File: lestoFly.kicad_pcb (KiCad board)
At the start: 2 copper layers, 23 x 29 mm, 24 parts, among them J1 Conn_01x02_Male, J2 Conn_01x15_Male, J5 Conn_Coaxial, U1 ESP32-WROOM-32D, U2 LMZM23601V3, U3 BMP280, U4 RFM95W-868S2, U5 BMX160

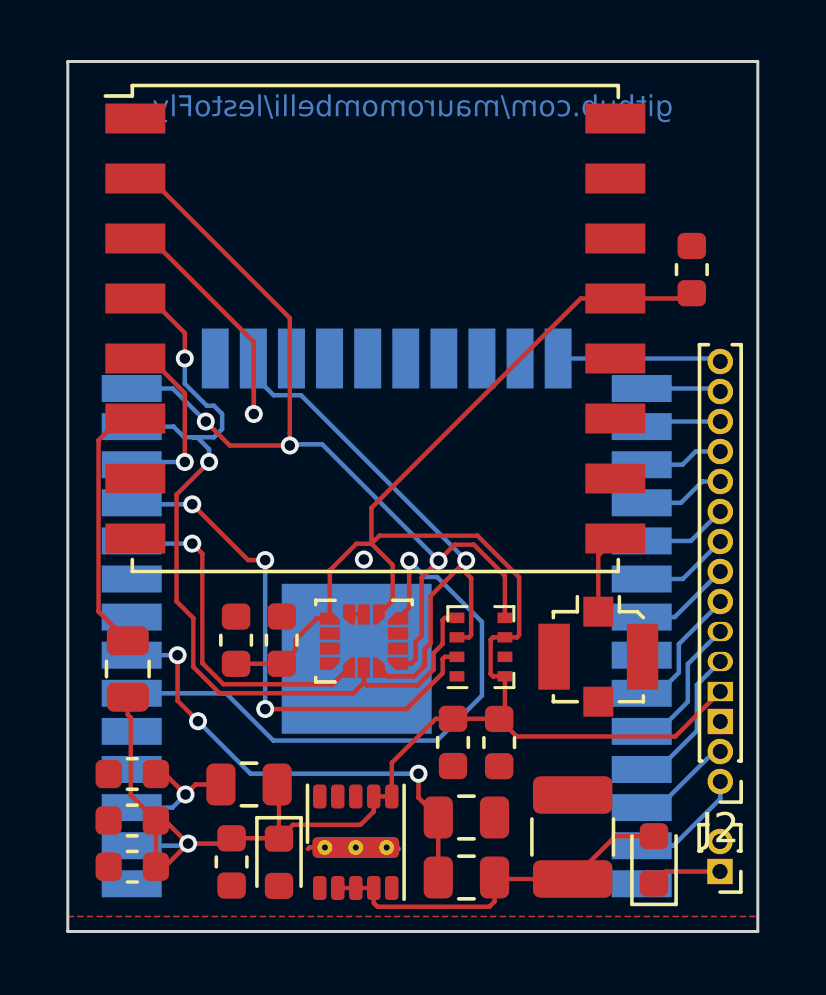
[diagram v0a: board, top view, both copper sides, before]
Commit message: completed the esp32 version
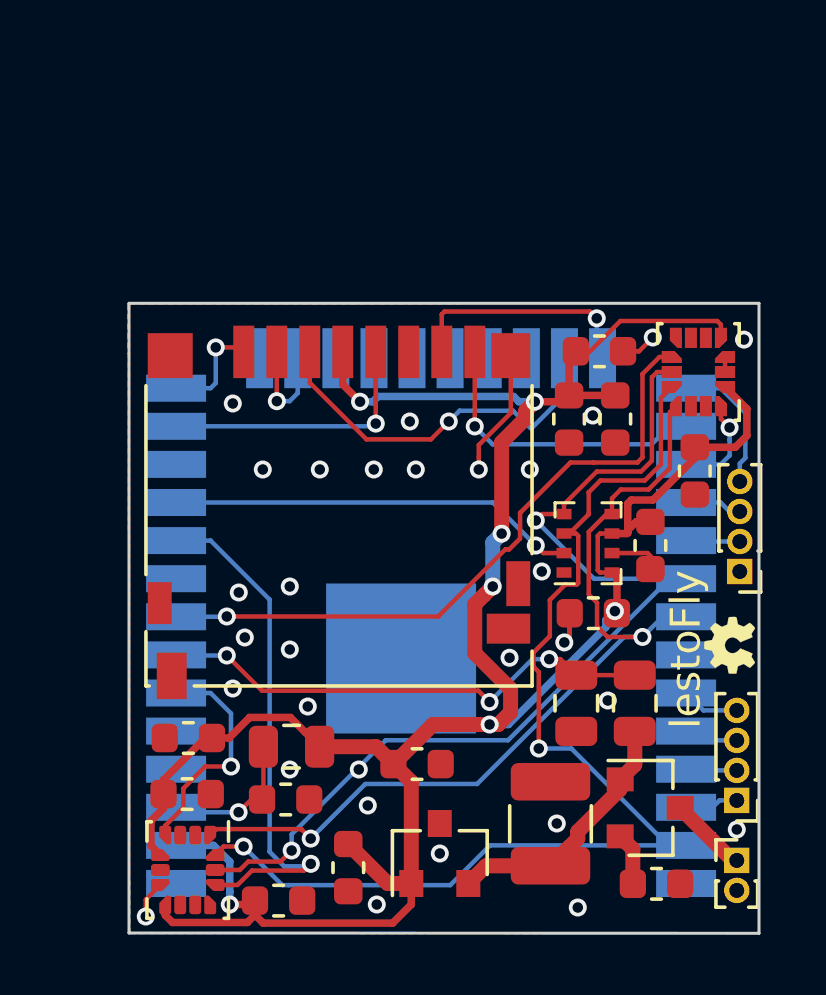
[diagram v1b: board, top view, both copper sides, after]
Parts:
- removed the C8 at (106.8, 46.9)
- removed D1: DIODE, Diode_SMD:D_0603_1608Metric
- removed D2: D_Zener, Diode_SMD:D_0603_1608Metric
- removed J2: Conn_01x15_Male, Connector_PinHeader_1.00mm:PinHeader_1x15_P1.00mm_Vertical
- removed R4: 10k, Resistor_SMD:R_0805_2012Metric
- removed U4: RFM95W-868S2, RF_Module:HOPERF_RFM9XW_SMD
- added C10: 100nF, Capacitor_SMD:C_0603_1608Metric, F.Cu at (93.0, 68.0)
- added C5: 100nF, Capacitor_SMD:C_0603_1608Metric, F.Cu at (104.2, 51.9)
- added C6: 10uF, Capacitor_SMD:C_0603_1608Metric, F.Cu at (102.7, 51.9)
- added C9: 100nF, Capacitor_SMD:C_0603_1608Metric, F.Cu at (90.0, 64.4)
- added G***: LOGO, lestoFly:oshw_2.0x1, F.Cu at (108.1, 59.5)
- added J3: Conn_01x04_Male, Connector_PinHeader_1.00mm:PinHeader_1x04_P1.00mm_Vertical, F.Cu at (108.3, 64.6)
- added J4: Conn_01x04_Male, lestoFly:PinHeader_1x04_P1.00mm_Vertical_small, F.Cu at (108.4, 57.0)
- added Q1: ZXMP6A13F, Package_TO_SOT_SMD:SOT-23, F.Cu at (105.4, 64.9)
- added R5: 12K, Capacitor_SMD:C_0603_1608Metric, F.Cu at (105.6, 67.4)
- added U6: BMX160, Package_LGA:LGA-14_3x2.5mm_P0.5mm_LayoutBorder3x4y, F.Cu at (90.0, 67.0)
- C13: renamed from C2; value 0.1uF -> 100nF
- C3: renamed from C4; value 10uF -> 0.1uF
- C4: renamed from C5; value 33uF -> 0.1uF
- J5: value Conn_Coaxial -> Micro_SD_Card_Det; footprint Connector_Coaxial:U.FL_Molex_MCRF_73412-0110_Vertical -> Connector_Card:microSD_HC_Hirose_DM3D-SF
- U2: value LMZM23601V3 -> LM3480-3.3; footprint Package_LGA:Texas_SIL0010A_MicroSiP-10-1EP_3.8x3mm_P0.6mm_EP0.7x2.9mm_ThermalVias -> Package_TO_SOT_SMD:SOT-23
- moved C11 15.5 mm to (103.7, 49.7), turned to 0 degrees
- moved C12 14.9 mm to (106.9, 53.6), turned to 270 degrees
- moved U5 14.3 mm to (107.0, 50.4), turned to 90 degrees
- moved J5 9.89 mm to (95.0, 55.0)
- moved C2 9.68 mm to (97.6, 63.4), turned to 0 degrees
- moved C8 8.28 mm to (105.4, 56.1)
- moved R2 8.08 mm to (104.9, 61.4), turned to 90 degrees
- moved C7 6.36 mm to (103.5, 58.4), turned to 180 degrees
- moved R3 5.28 mm to (103.0, 61.4), turned to 270 degrees
- moved C13 5.18 mm to (93.3, 64.6), turned to 0 degrees
- moved U3 4.97 mm to (103.3, 56.1)
- moved C1 4.68 mm to (90.0, 62.5)
- moved C4 3.89 mm to (95.3, 66.9)
- moved U2 2.83 mm to (98.4, 66.4)
- moved R1 1.89 mm to (93.5, 62.8)
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- renumbered C7 to C11, C10 to C12, C3 to C2, C6 to C7, C9 to C8
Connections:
- J5 pad 1: Net-(J5-Pad1) -> SD_DAT2
- J5 pad 2: GND -> SD_DAT3
- U1 pad 10: CS_IMU -> CS_IMU_1
- U1 pad 12: CS_LORA -> Net-(U1-Pad12)
- U1 pad 13: CLK -> SD_CLK
- U1 pad 14: MISO -> SD_DAT2
- U1 pad 16: MOSI -> SD_DAT3
- U1 pad 23: Net-(U1-Pad23) -> SD_CMD
- U1 pad 24: 15 -> SD_DAT0
- U1 pad 25: 14 -> 7
- U1 pad 26: 13 -> SD_DAT1
- U1 pad 27: 12 -> INT_IMU_2
- U1 pad 28: 11 -> 6
- U1 pad 29: 10 -> 5
- U1 pad 30: 9 -> CLK
- U1 pad 31: 8 -> MISO
- U1 pad 33: 7 -> 4
- U1 pad 34: 6 -> 3
- U1 pad 35: 5 -> 2
- U1 pad 36: 2 -> 1
- U1 pad 37: 1 -> MOSI
- U1 pad 6: INT_IMU -> INT_IMU_1
- U1 pad 8: Net-(U1-Pad8) -> CS_IMU_2
- U2 pad 1: GND -> +3V3
- U2 pad 3: VCC -> GND
- U5 pad 12: CS_IMU -> CS_IMU_2
- U5 pad 4: INT_IMU -> INT_IMU_2
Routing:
- net CS_IMU_2: track 0.00 -> 22.2 mm, vias 0 -> 1
- net INT_IMU: track 20.8 -> 0.00 mm, vias 1 -> 0
- net CS_IMU_1: track 0.00 -> 17.4 mm, vias 0 -> 1
- net +3V3: track 70.8 -> 87.9 mm, vias 1 -> 7
- net SD_CMD: track 0.00 -> 12.6 mm, vias 0 -> 1
- net CS_IMU: track 11.6 -> 0.00 mm, vias 1 -> 0
- net MOSI: track 28.8 -> 39.0 mm
- net SD_DAT1: track 0.00 -> 10.0 mm, vias 0 -> 1
- net SD_CLK: track 0.00 -> 9.08 mm, vias 0 -> 1
- net Net-(R4-Pad1): track 8.62 -> 0.00 mm
- net SD_DAT0: track 0.00 -> 7.96 mm, vias 0 -> 1
- net INT_IMU_1: track 0.00 -> 7.58 mm, vias 0 -> 1
- net GND: track 3.58 -> 10.8 mm, vias 1 -> 29
- net CS_LORA: track 6.23 -> 0.00 mm, vias 1 -> 0
- net 15: track 5.45 -> 0.00 mm
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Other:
- board size 23 x 29 mm -> 21 x 21 mm
- board text added: "lestoFly"
- board text removed: "github.com/mauromombelli/lestoFly"
